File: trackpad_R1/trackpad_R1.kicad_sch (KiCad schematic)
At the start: 17 parts, among them J1 Conn_01x17

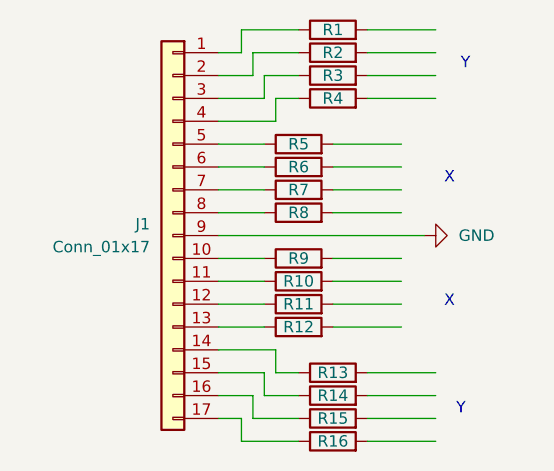
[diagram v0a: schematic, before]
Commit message: progress
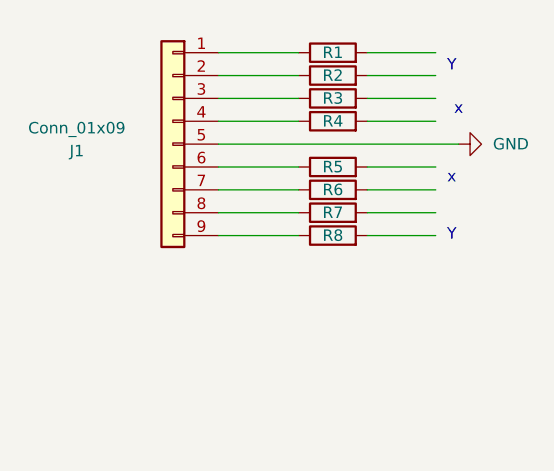
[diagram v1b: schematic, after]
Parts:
- removed J1: Conn_01x17, Connector_PinHeader_2.54mm:PinHeader_1x17_P2.54mm_Horizontal, symbol Connector_Generic:Conn_01x17
- removed R10, R11, R12, R13, R14, R15, R16, R9: R, Resistor_SMD:R_1206_3216Metric_Pad1.30x1.75mm_HandSolder, symbol Device:R
- added J1: Conn_01x09, Connector_PinHeader_2.54mm:PinHeader_1x09_P2.54mm_Horizontal, symbol Connector_Generic:Conn_01x09
- R1, R2, R3, R4, R5, R6, R7: footprint Resistor_SMD:R_1206_3216Metric_Pad1.30x1.75mm_HandSolder -> Library:R_1206_3216Metric_Pad1.30x1.75mm_HandSolder_extra
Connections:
- net GND: now also J1.5 (Pin_5)
- net at R3.1: now also J1.3 (Pin_3)
- net at R1.1: now also J1.1 (Pin_1)
- net at R8.1: now also J1.9 (Pin_9)
- net at R7.1: now also J1.8 (Pin_8)
- net at R4.1: now also J1.4 (Pin_4)
- net at R6.1: now also J1.7 (Pin_7)
- net at R2.1: now also J1.2 (Pin_2)
- net at R5.1: now also J1.6 (Pin_6)
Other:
- note added: "x"
- note removed: "X"
- moved on the sheet: R5, R8
